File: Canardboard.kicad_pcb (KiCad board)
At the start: 4 copper layers, 50 x 58.5 mm, 164 parts, among them IC1 SIC437DED-T1-GE3, J1 RBUS, J2 USB_C_Receptacle_USB2.0, J3 Micro_SD_Card_Det, J4 Conn_01x02_Male, J5 Conn_01x03_Male, J6 Conn_01x03_Male, J7 Conn_01x03_Male, Q1 PXP012-30QLJ, Q2 PXP012-30QLJ, Q4 PXP012-30QLJ, Q6 PXP012-30QLJ, U1 ESP32-S3, U10 MP28167GQ-A-Z, U2 SN65HVD230, U3 LTC4412xS6, U4 LTC4412xS6, U5 74AHC1G00, U6 74AHC1G08, U7 ICM-20608-G, U8 MMC5983MA, Y1 40MHz±10ppm

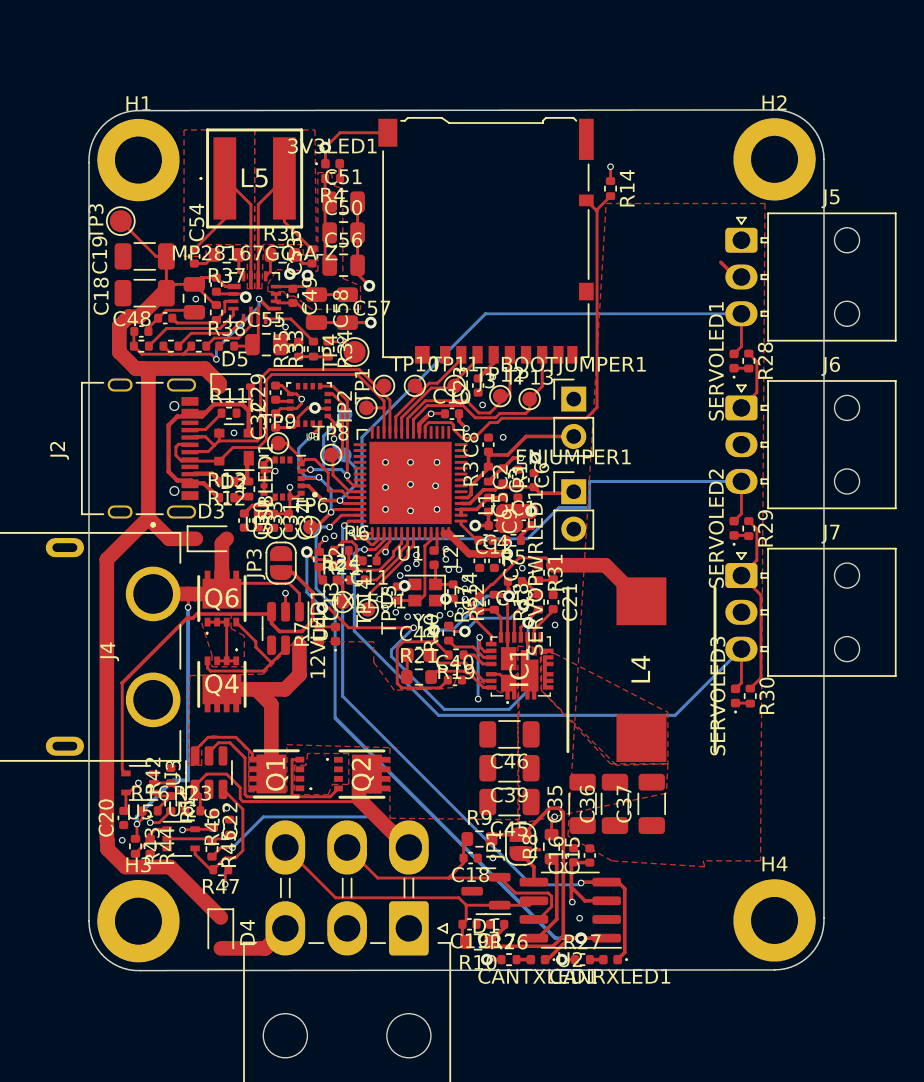
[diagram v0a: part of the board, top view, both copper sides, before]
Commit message: fixed all of andrei's comments v1
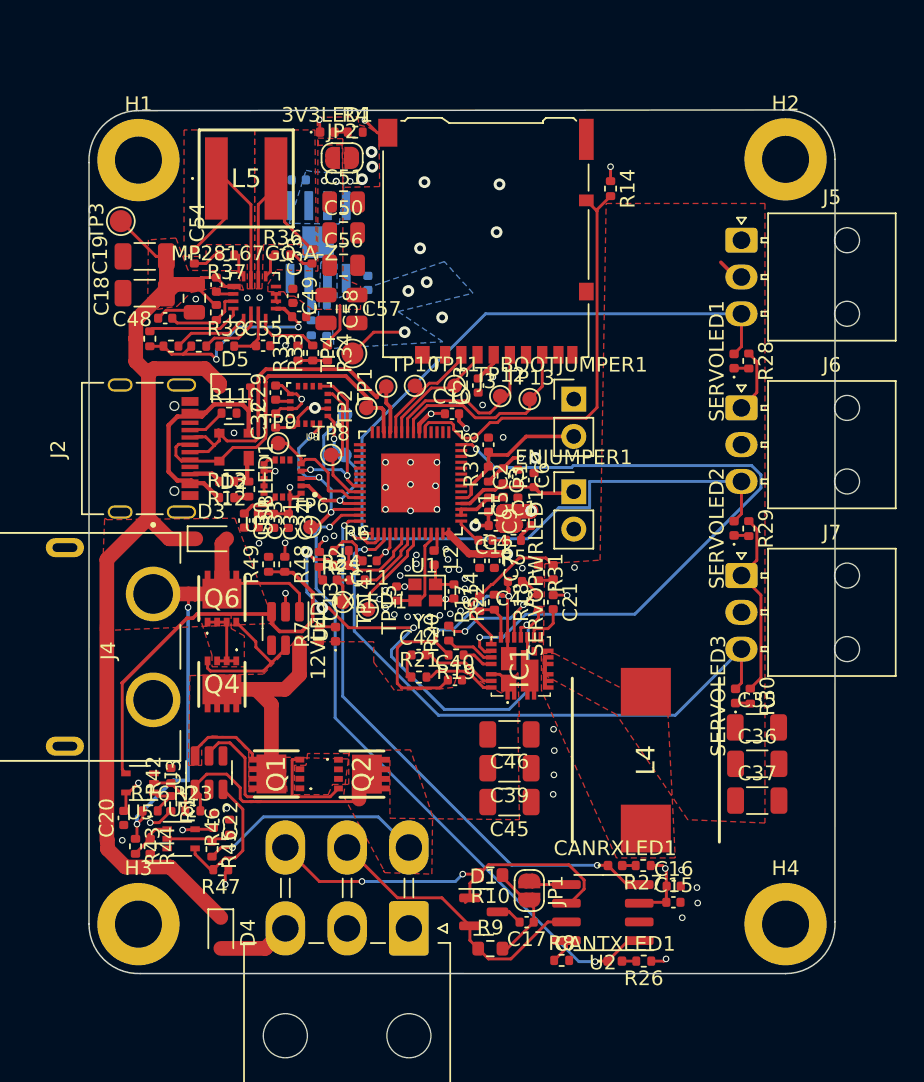
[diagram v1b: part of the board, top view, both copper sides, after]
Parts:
- removed the C18 at (126.6, 122.5)
- removed the C19 at (126.5, 127.0)
- removed JP3: SolderJumper_2_Open, Jumper:SolderJumper-2_P1.3mm_Open_RoundedPad1.0x1.5mm
- added C24: DNP, Capacitor_SMD:C_0402_1005Metric, B.Cu at (114.9, 76.4)
- added C25: DNP, Capacitor_SMD:C_0402_1005Metric, B.Cu at (119.6, 83.4)
- added C26: 0.1uF, Capacitor_SMD:C_0402_1005Metric, B.Cu at (116.8, 86.5)
- added JP2: TermJP, Jumper:SolderJumper-2_P1.3mm_Open_RoundedPad1.0x1.5mm, F.Cu at (117.8, 74.9)
- added R48: 100k, Resistor_SMD:R_0402_1005Metric, F.Cu at (114.0, 102.5)
- added R49: 0, Resistor_SMD:R_0402_1005Metric, F.Cu at (112.8, 102.5)
- added R50: DNP, Resistor_SMD:R_0402_1005Metric, B.Cu at (116.3, 84.9)
- added R51: DNP, Resistor_SMD:R_0402_1005Metric, B.Cu at (115.8, 86.5)
- added U9: SC4215, iclr:SOIC127P599X175-9N, B.Cu at (116.2, 80.6)
- C44: footprint Capacitor_SMD:C_0603_1608Metric -> Capacitor_SMD:C_0402_1005Metric
- C55: footprint Capacitor_SMD:C_0805_2012Metric -> Capacitor_SMD:C_0402_1005Metric
- R15, R42, R44, R46: value 570 -> 470
- R16, R23, R43, R45: value 1.5k -> 1k
- R21, R36, R37, R8: footprint Resistor_SMD:R_0603_1608Metric -> Resistor_SMD:R_0402_1005Metric
- U1: footprint Package_DFN_QFN:QFN-56-1EP_7x7mm_P0.4mm_EP5.6x5.6mm -> iclr:QFN40P700X700X90-57N
- moved C35 12.9 mm to (146.1, 113.6), turned to 0 degrees
- moved C52 10.8 mm to (114.9, 85.7)
- moved C36 10.1 mm to (146.1, 116.1), turned to 0 degrees
- moved R26 9.16 mm to (138.4, 129.5), turned to 180 degrees
- moved R8 7.76 mm to (132.8, 129.5), turned to 0 degrees
- moved R27 7.62 mm to (138.3, 123.0), turned to 180 degrees
- moved R9 7.49 mm to (127.9, 128.7)
- moved C37 7.18 mm to (146.1, 118.6), turned to 0 degrees
- moved C16 7.12 mm to (140.4, 124.4), turned to 0 degrees
- moved C15 6.52 mm to (140.4, 125.5), turned to 0 degrees
- moved CANRXLED1 6.41 mm to (136.4, 123.0), turned to 0 degrees
- moved L4 6.16 mm to (138.5, 115.8)
- moved CANTXLED1 5.23 mm to (136.4, 129.5), turned to 0 degrees
- moved R10 4.62 mm to (127.9, 123.7)
- moved R4 3.51 mm to (118.7, 73.2), turned to 0 degrees
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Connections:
- C49 pad 1: +3.3V -> /servopower/uC_VOUT
- C50 pad 1: +3.3V -> /servopower/uC_VOUT
- C51 pad 1: +3.3V -> /servopower/uC_VOUT
- C56 pad 1: +3.3V -> /servopower/uC_VOUT
- C57 pad 1: +3.3V -> /servopower/uC_VOUT
- C58 pad 1: +3.3V -> /servopower/uC_VOUT
- IC1 pad 19: +12V -> /SERVOBUCK_EN
- R34 pad 1: +3.3V -> /servopower/uC_VOUT
- U1 pad 14: unconnected-(U1-GPIO9/ADC1_CH8-Pad14) -> /SERVOBUCK_EN
- U10 pad 12: +3.3V -> /servopower/uC_VOUT
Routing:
- net /SERVOBUCK_EN: track 0.00 -> 47.4 mm, vias 0 -> 2
- net GND: track 72.2 -> 54.8 mm, vias 56 -> 69
- net Net-(JP1-B): track 21.2 -> 7.11 mm
- net +3.3V: track 60.4 -> 49.6 mm, vias 19 -> 23
- net /SERVO_PWR: track 18.8 -> 11.8 mm
- net +12V: track 26.8 -> 20.8 mm, vias 2 -> 0
- net /CAN-: track 21.4 -> 26.8 mm, vias 0 -> 2
- net /rbusmosfets/RBUS_DEPL: track 37.1 -> 32.4 mm
- net Net-(U2-Rs): track 6.34 -> 1.69 mm
- net /CAN_RX: track 42.6 -> 38.4 mm
- net /servopower/uC_VOUT: track 0.00 -> 3.51 mm, vias 0 -> 2
- net Net-(U9-ADJ): track 0.00 -> 3.05 mm
- net /Data-: track 24.1 -> 25.6 mm
- net RBUS_uC_V: track 75.7 -> 74.2 mm
- net Net-(U4-CTL): track 27.2 -> 28.3 mm
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- added copper zone on B.Cu, net +3.3V
- added copper zone on F.Cu, net /rbusmosfets/BatteryPower
- added copper zone on F.Cu, net /rbusmosfets/RBUS_DEPL
- added copper zone on B.Cu, net /servopower/uC_VOUT
- added copper zone on F.Cu, net /servopower/uC_VOUT
- added copper zone on F.Cu, net RBUS_uC_V
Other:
- board size 50 x 58.5 mm -> 50.7 x 58.7 mm
